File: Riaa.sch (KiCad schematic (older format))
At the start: 46 parts, among them J1 +15V, J2 GND, J3 -15V, J4 +IN, J5 GND, U1 TL071, U2 TL072, U3 TL071, U4 TL071

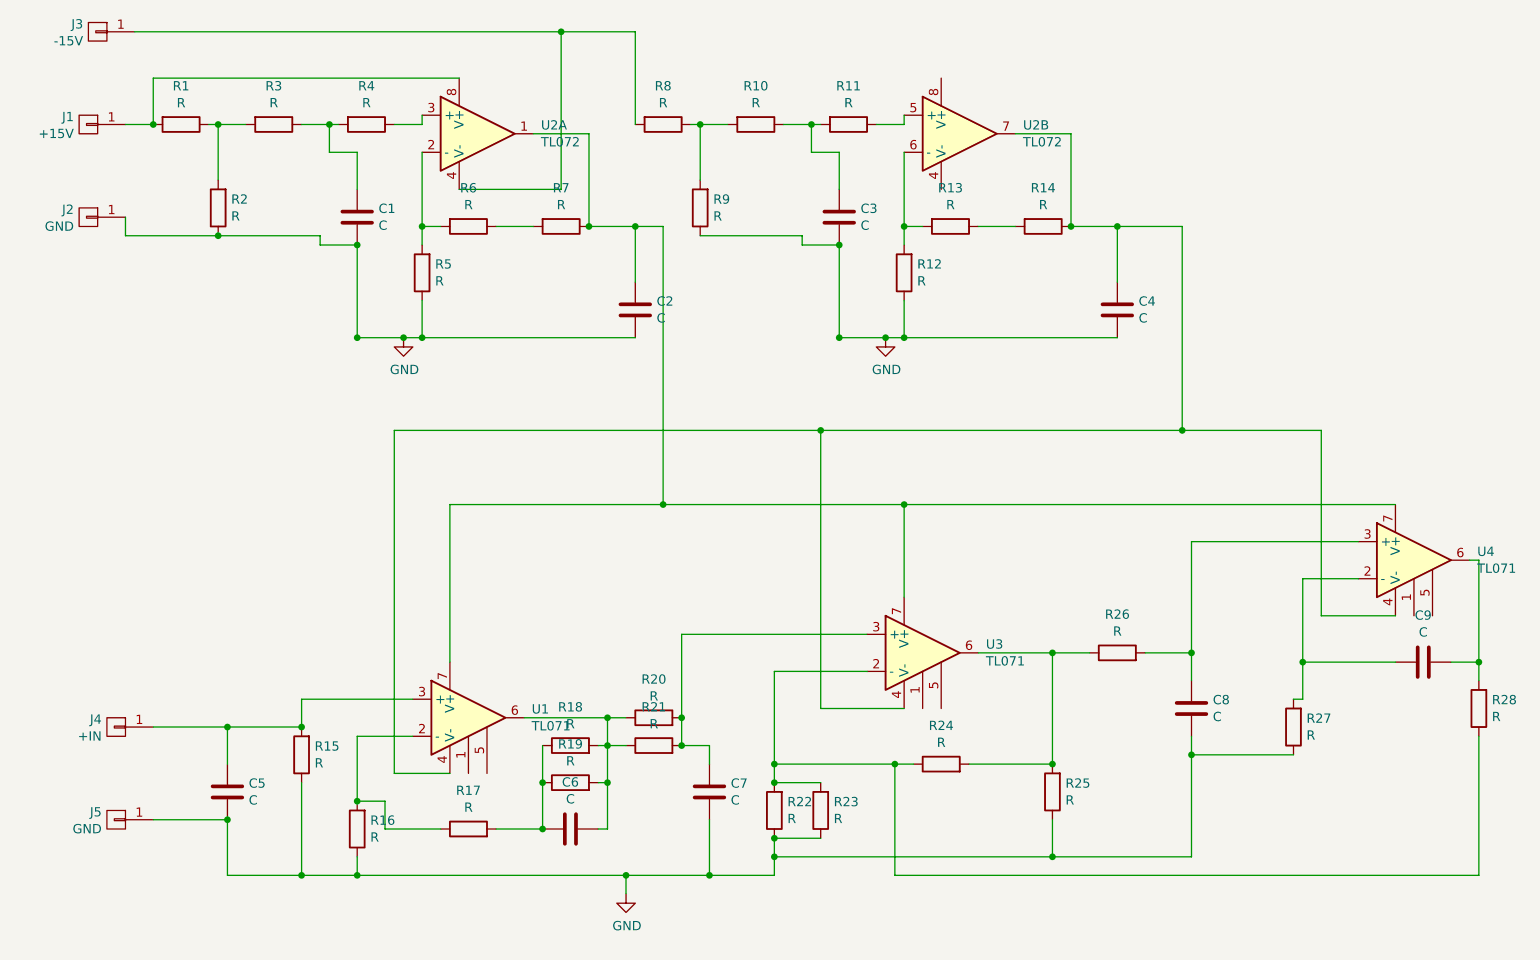
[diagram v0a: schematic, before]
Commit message: component values
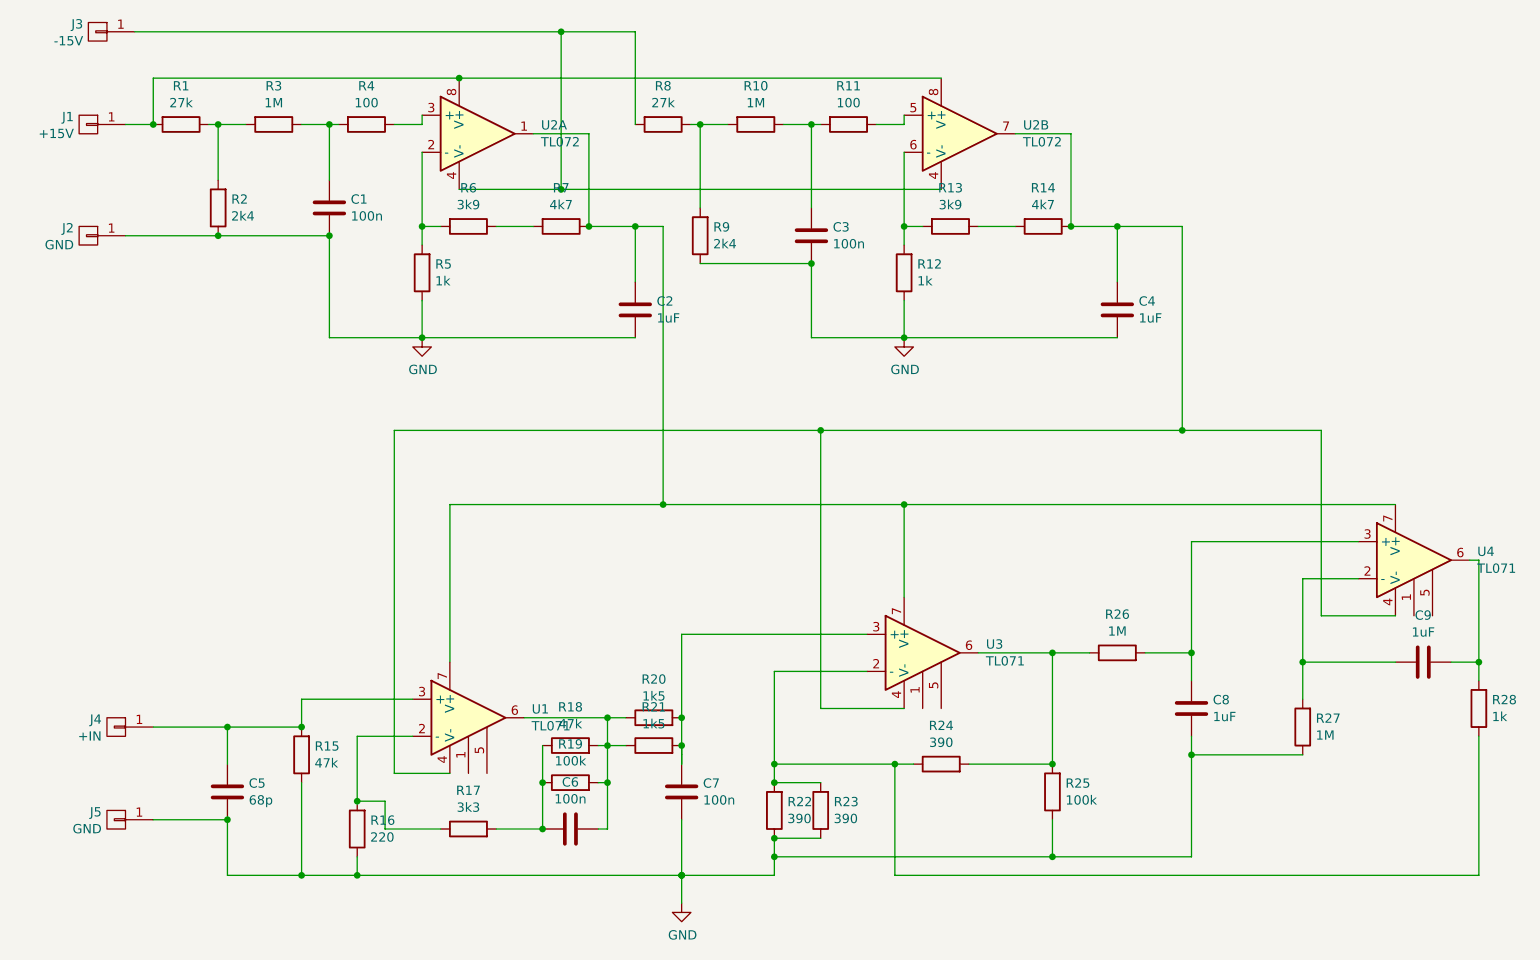
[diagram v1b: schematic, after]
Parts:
- C1, C3, C6, C7: value C -> 100n
- C2, C4, C8, C9: value C -> 1uF
- C5: value C -> 68p
- R1, R8: value R -> 27k
- R10, R26, R27, R3: value R -> 1M
- R11, R4: value R -> 100
- R12, R28, R5: value R -> 1k
- R13, R6: value R -> 3k9
- R14, R7: value R -> 4k7
- R15, R18: value R -> 47k
- R16: value R -> 220
- R17: value R -> 3k3
- R19, R25: value R -> 100k
- R2, R9: value R -> 2k4
- R20, R21: value R -> 1k5
- R22, R23, R24: value R -> 390
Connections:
- net at J3.1 (P1), R8.2, U2.4 (V-): now also U2.4 (V-)
- net at J1.1 (P1), R1.2, U2.8 (V+): now also U2.8 (V+)
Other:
- moved on the sheet: C1, C3, C7, J2, R27, R9

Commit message: pads
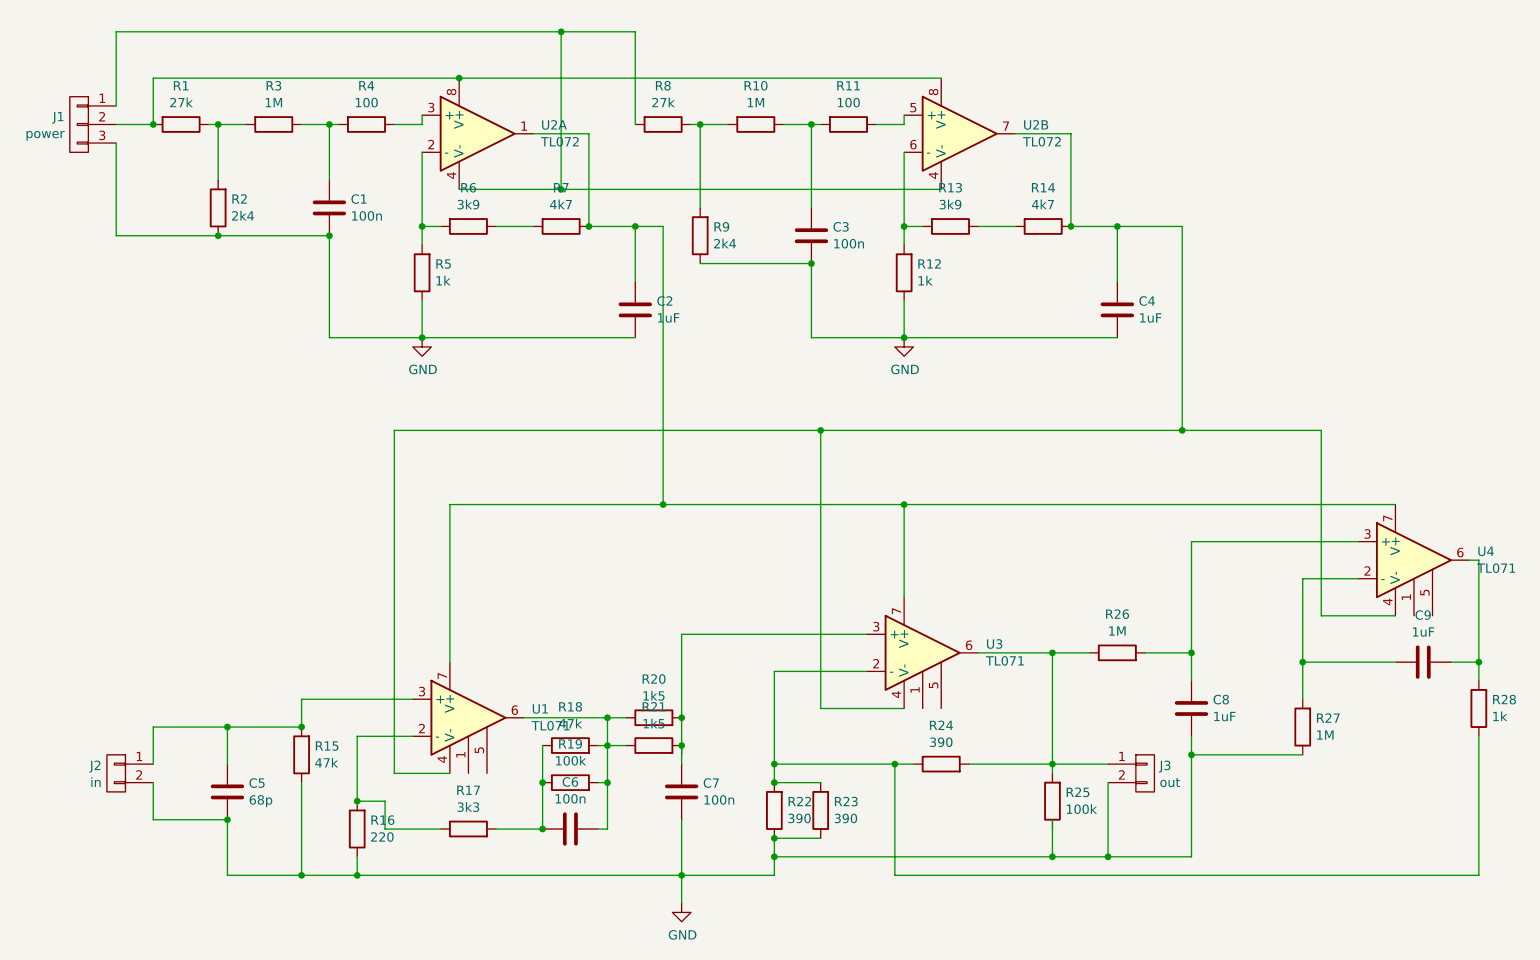
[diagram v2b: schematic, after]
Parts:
- removed J1: +15V, symbol CONN_01X01
- removed J2, J5: GND, symbol CONN_01X01
- removed J3: -15V, symbol CONN_01X01
- removed J4: +IN, symbol CONN_01X01
- added J1: power, Connectors:PINHEAD1-3, symbol CONN_01X03
- added J2: in, Connectors:PINHEAD1-2, symbol CONN_01X02
- added J3: out, Connectors:PINHEAD1-2, symbol CONN_01X02
- C1, C3, C5, C6, C7: footprint (none) -> Capacitors_THT:C_Rect_L7.2mm_W2.5mm_P5.00mm_FKS2_FKP2_MKS2_MKP2
- C2, C4, C8, C9: footprint (none) -> Capacitors_THT:C_Rect_L7.2mm_W5.5mm_P5.00mm_FKS2_FKP2_MKS2_MKP2
- R1, R10, R11, R12, R13, R14, R15, R16, R17, R18, R19, R2, R20, R21, R22, R23, R24, R25, R26, R27, R28, R3, R4, R5, R6, R7, R8, R9: footprint (none) -> Resistors_THT:R_Axial_DIN0207_L6.3mm_D2.5mm_P7.62mm_Horizontal
- U1, U2, U3, U4: footprint (none) -> Housings_DIP:DIP-8_W7.62mm
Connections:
- net GND: now also J1.3 (P3), J2.2 (P2), J3.2 (P2); no longer R25.1
- net at R8.2, U2.4 (V-), U2.4 (V-): now also J1.1 (P1)
- net at R1.2, U2.8 (V+), U2.8 (V+): now also J1.2 (P2)
- net at C5.1, R15.2, U1.3 (+): now also J2.1 (P1)
- net at R24.2, R25.2, R26.1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: now also J3.1 (P1)
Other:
- moved on the sheet: R25

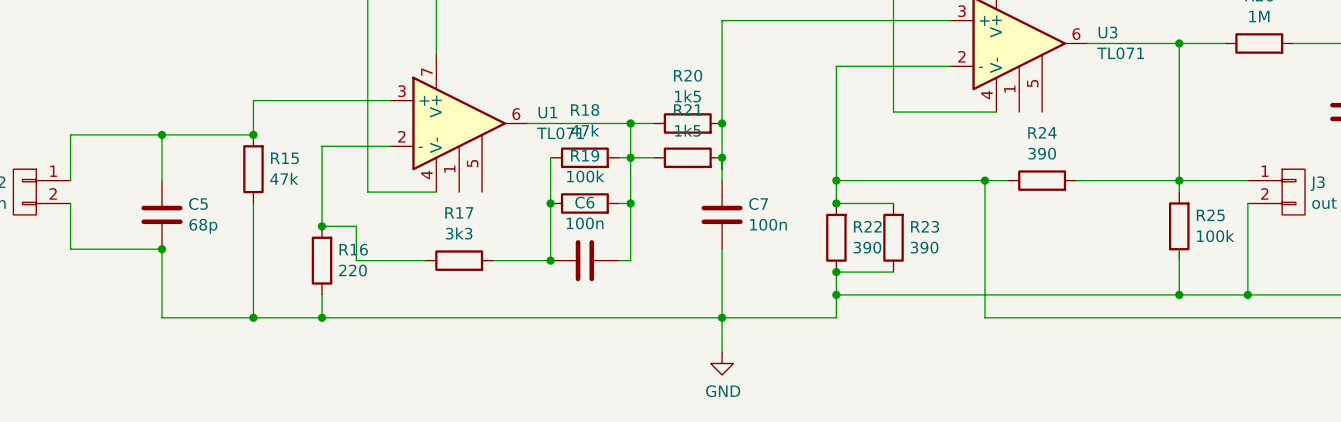
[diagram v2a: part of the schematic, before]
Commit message: layout
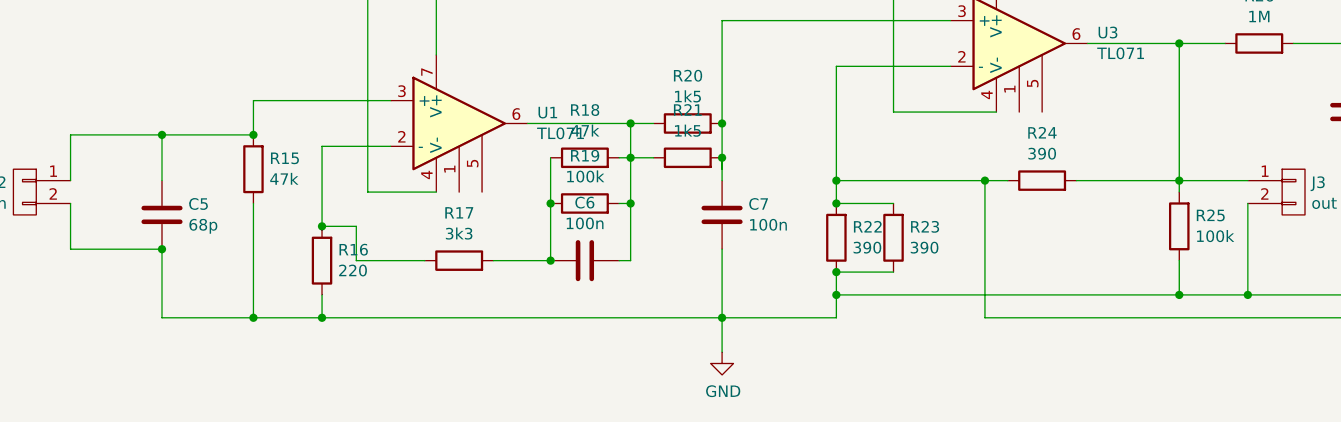
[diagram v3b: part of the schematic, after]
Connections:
- net GND: now also R25.1
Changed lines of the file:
@@
 	1900 5800 1900 6100
 Wire Wire Line
-	1900 6100 4850 6100
+	4850 6100 1900 6100
 Wire Wire Line
 	2300 6100 2300 5600
@@
 	5900 5500 6650 5500
 Wire Wire Line
-	6350 5800 6350 6000
+	6350 5850 6350 6000
 Wire Wire Line
 	7100 6000 4850 6000
